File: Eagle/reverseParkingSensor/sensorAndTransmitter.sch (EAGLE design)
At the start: 29 parts, among them IC1 LM393N, IC3 MEGA8-P, Q1 BC558B, T1 BPX81, X1 YH-55-10

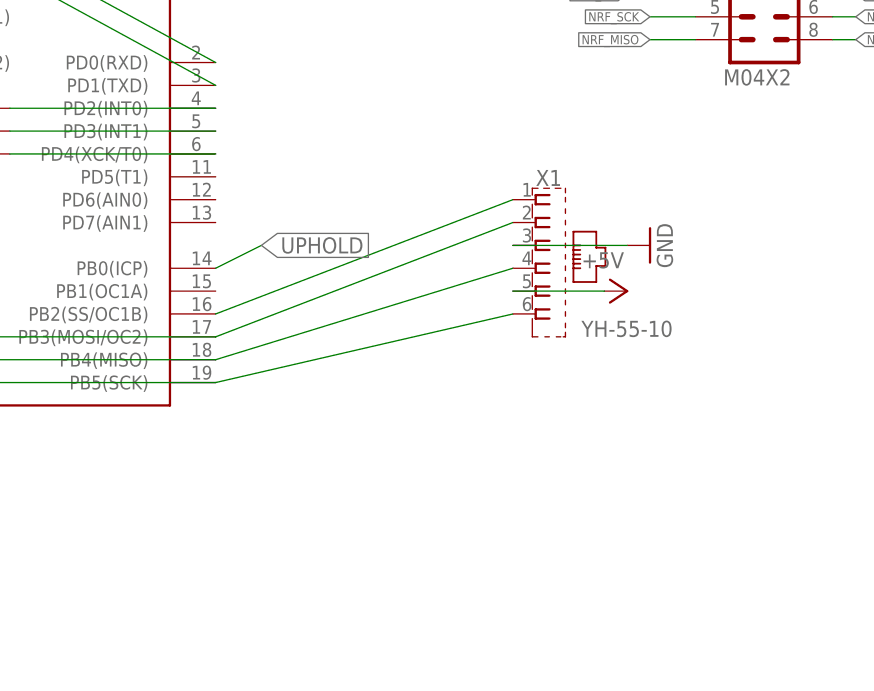
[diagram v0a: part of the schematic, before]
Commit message: final pcb for sensor and transmitter
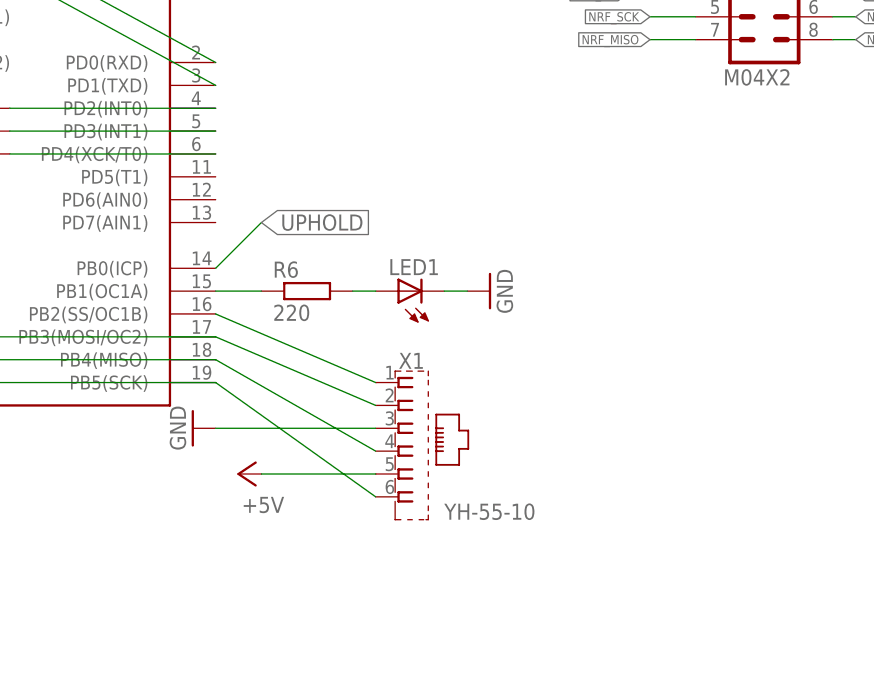
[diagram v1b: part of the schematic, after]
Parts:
- added LED1: (no value), led:LED3MM
- added R6: 220, resistor:R-EU_0207/10
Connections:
- new net N$6: IC3.PB1(OC1A), R6.1
- new net N$7: LED1.A, R6.2
- net GND: now also LED1.C
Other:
- moved on the sheet: X1
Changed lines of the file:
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@@
 <part name="P+1" library="supply1" deviceset="+5V" device=""/>
 <part name="Q1" library="transistor-pnp" deviceset="BC558*" device="" technology="B"/>
+<part name="LED1" library="led" deviceset="LED" device="3MM"/>
+<part name="R6" library="resistor" deviceset="R-EU_" device="0207/10" value="220"/>
+<part name="GND1" library="supply1" deviceset="GND" device=""/>
 </parts>
 <sheets>
@@
 <instance part="JP4" gate="1" x="190.5" y="86.36" rot="R270"/>
 <instance part="JP5" gate="1" x="190.5" y="63.5" rot="R90"/>
-<instance part="GND18" gate="1" x="264.16" y="50.8" rot="R90"/>
-<instance part="X1" gate="G$1" x="256.54" y="48.26"/>
-<instance part="P+1" gate="1" x="261.62" y="45.72" rot="R270"/>
+<instance part="GND18" gate="1" x="213.36" y="30.48" rot="R270"/>
+<instance part="X1" gate="G$1" x="241.3" y="27.94"/>
+<instance part="P+1" gate="1" x="218.44" y="25.4" rot="R90"/>
 <instance part="Q1" gate="G$1" x="-30.48" y="35.56" rot="R180"/>
+<instance part="LED1" gate="G$1" x="236.22" y="45.72" rot="R90"/>
+<instance part="R6" gate="G$1" x="226.06" y="45.72"/>
+<instance part="GND1" gate="1" x="246.38" y="45.72" rot="R90"/>
 </instances>
 <busses>
@@
 <pinref part="P+1" gate="1" pin="+5V"/>
 <pinref part="X1" gate="G$1" pin="5"/>
-<wire x1="259.08" y1="45.72" x2="248.92" y2="45.72" width="0.1524" layer="91"/>
+<wire x1="220.98" y1="25.4" x2="233.68" y2="25.4" width="0.1524" layer="91"/>
 </segment>
 </net>
@@
 <pinref part="GND18" gate="1" pin="GND"/>
 <pinref part="X1" gate="G$1" pin="3"/>
-<wire x1="261.62" y1="50.8" x2="248.92" y2="50.8" width="0.1524" layer="91"/>
+<wire x1="215.9" y1="30.48" x2="233.68" y2="30.48" width="0.1524" layer="91"/>
+</segment>
+<segment>
+<pinref part="GND1" gate="1" pin="GND"/>
+<pinref part="LED1" gate="G$1" pin="C"/>
+<wire x1="243.84" y1="45.72" x2="241.3" y2="45.72" width="0.1524" layer="91"/>
 </segment>
 </net>
@@
 <segment>
 <pinref part="IC3" gate="G$1" pin="PB0(ICP)"/>
-<wire x1="215.9" y1="48.26" x2="220.98" y2="50.8" width="0.1524" layer="91"/>
-<label x="220.98" y="50.8" size="1.778" layer="95" xref="yes"/>
+<wire x1="215.9" y1="48.26" x2="220.98" y2="53.34" width="0.1524" layer="91"/>
+<label x="220.98" y="53.34" size="1.778" layer="95" xref="yes"/>
 </segment>
 </net>
@@
 <wire x1="215.9" y1="40.64" x2="187.96" y2="40.64" width="0.1524" layer="91"/>
 <pinref part="X1" gate="G$1" pin="2"/>
-<wire x1="215.9" y1="40.64" x2="248.92" y2="53.34" width="0.1524" layer="91"/>
+<wire x1="215.9" y1="40.64" x2="233.68" y2="33.02" width="0.1524" layer="91"/>
 </segment>
 </net>
@@
 <wire x1="215.9" y1="35.56" x2="187.96" y2="35.56" width="0.1524" layer="91"/>
 <pinref part="X1" gate="G$1" pin="6"/>
-<wire x1="215.9" y1="35.56" x2="248.92" y2="43.18" width="0.1524" layer="91"/>
+<wire x1="215.9" y1="35.56" x2="233.68" y2="22.86" width="0.1524" layer="91"/>
 </segment>
 </net>
@@
 <wire x1="215.9" y1="38.1" x2="187.96" y2="38.1" width="0.1524" layer="91"/>
 <pinref part="X1" gate="G$1" pin="4"/>
-<wire x1="215.9" y1="38.1" x2="248.92" y2="48.26" width="0.1524" layer="91"/>
+<wire x1="215.9" y1="38.1" x2="233.68" y2="27.94" width="0.1524" layer="91"/>
 </segment>
 </net>
@@
 <pinref part="IC3" gate="G$1" pin="PB2(SS/OC1B)"/>
 <pinref part="X1" gate="G$1" pin="1"/>
-<wire x1="215.9" y1="43.18" x2="248.92" y2="55.88" width="0.1524" layer="91"/>
-</segment>
-</net>
+<wire x1="215.9" y1="43.18" x2="233.68" y2="35.56" width="0.1524" layer="91"/>
+</segment>
+</net>
+<net name="N$6" class="0">
+<segment>
+<pinref part="IC3" gate="G$1" pin="PB1(OC1A)"/>
+<pinref part="R6" gate="G$1" pin="1"/>
+<wire x1="220.98" y1="45.72" x2="215.9" y2="45.72" width="0.1524" layer="91"/>
+</segment>
+</net>
+<net name="N$7" class="0">
+<segment>
+<pinref part="R6" gate="G$1" pin="2"/>
+<pinref part="LED1" gate="G$1" pin="A"/>
+<wire x1="231.14" y1="45.72" x2="233.68" y2="45.72" width="0.1524" layer="91"/>
+</segment>
+</net>
